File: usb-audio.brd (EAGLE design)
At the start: 100 x 80 mm, 12 parts

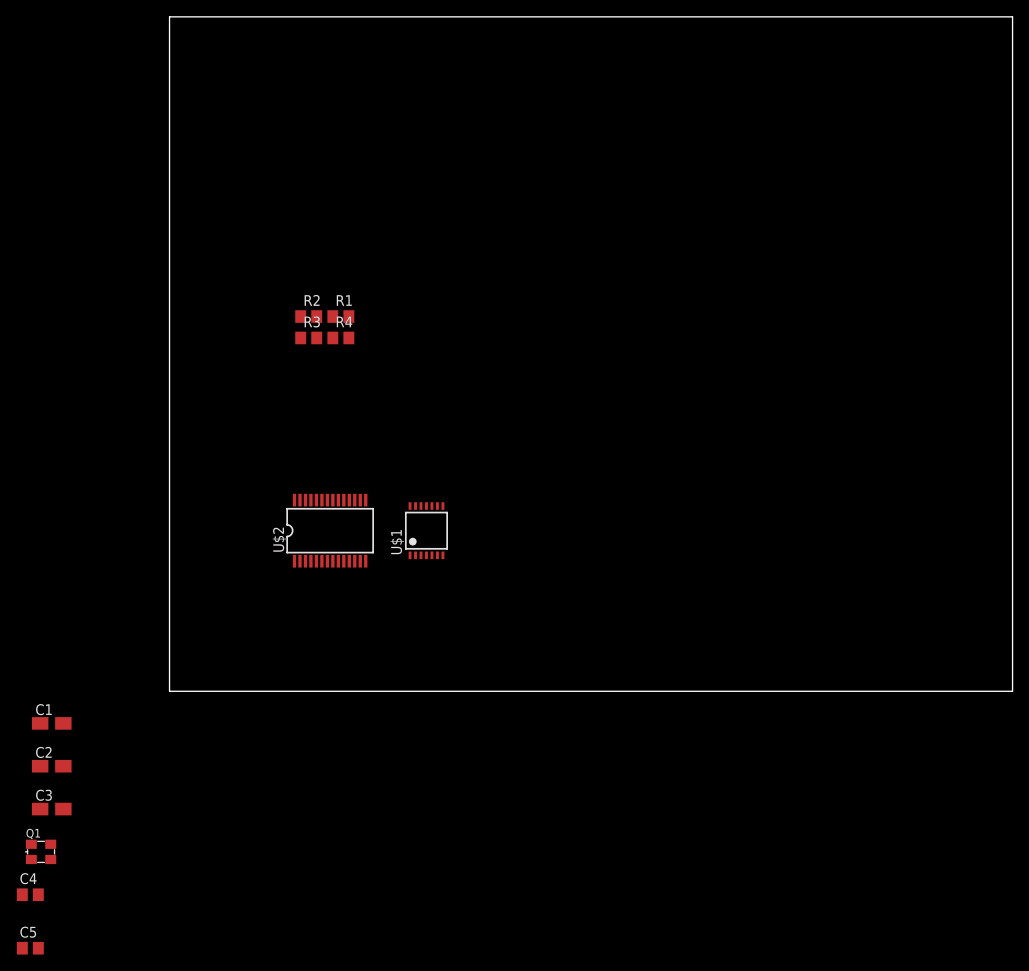
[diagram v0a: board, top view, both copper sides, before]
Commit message: .
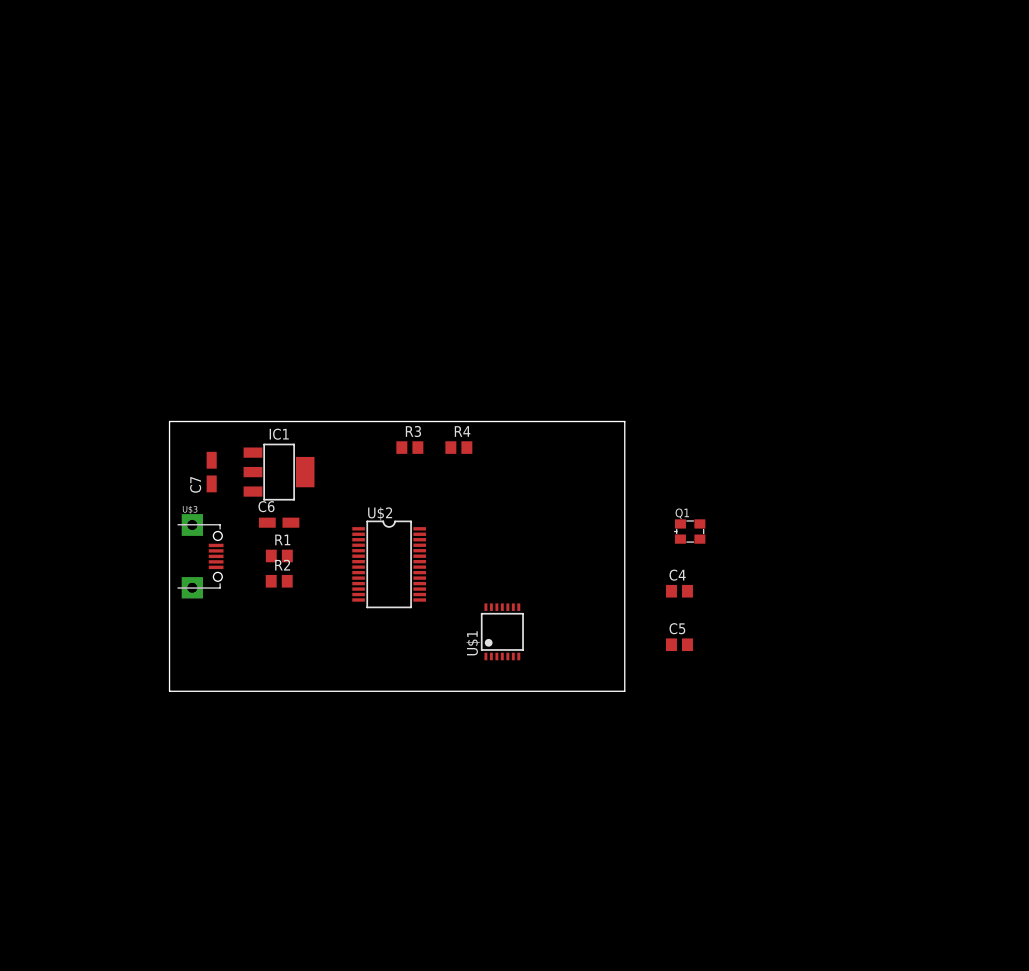
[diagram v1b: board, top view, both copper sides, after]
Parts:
- removed C1, C2, C3: (no value), rcl:A/3216-18R
- added C6: 10mF, rcl:CT3216
- added C7: 100mF, rcl:CT3216
- added IC1: LM1117MPX-3.3, lm1117:SOT223
- added U$3: MICRO-USB, microusb:MICRO-USB
- moved Q1 85.9 mm to (61.8, 18.9)
- moved C4 85.0 mm to (60.5, 11.9)
- moved C5 85.0 mm to (60.5, 5.52)
- moved R2 31.6 mm to (13.0, 13.1)
- moved R1 29.3 mm to (13.0, 16.1)
- moved R4 19.1 mm to (34.3, 28.9)
- moved R3 17.7 mm to (28.5, 28.9)
- moved U$1 15.0 mm to (39.5, 7.05)
- moved U$2 8.06 mm to (26.1, 15.1), turned to 270 degrees
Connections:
- removed net SVSS: U$1.12
- removed net VDD: U$1.2
- new net +3V3: C7.+, IC1.2, IC1.TAB
- new net AGND: U$1.10, U$1.4, U$2.12, U$2.17
- new net GND: C4.2, C5.2, C6.-, C7.-, IC1.1, U$3.5, U$3.GND1, U$3.GND2
- new net N$10: U$1.5
- new net N$11: U$1.9, U$2.14
- new net N$12: U$1.11, U$2.15
- new net N$13: U$1.12, U$1.7
- new net N$5: R1.1, U$3.2
- new net N$6: R2.1, U$3.3
- new net N$7: C5.1, Q1.1, U$2.28
- new net N$8: C4.1, Q1.3, U$2.1
- new net N$9: U$1.3
- new net VCC: C6.+, IC1.3, U$1.2, U$1.8, U$3.1
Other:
- board size 100 x 80 mm -> 54 x 32 mm
